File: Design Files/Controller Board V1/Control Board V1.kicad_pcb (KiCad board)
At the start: 4 copper layers, 75 x 125 mm, 78 parts, among them J1 XT30PW-F, J10 SM04B-GHS-TB_LF__SN_-, J11 SM04B-GHS-TB_LF__SN_-, J2 XT30UPB-M, J3 XT30UPB-M, J4 XT30UPB-M, J5 XT30UPB-M, J6 XT30UPB-M, J7 XT30UPB-M, J8 SM04B-GHS-TB_LF__SN_-, J9 SM04B-GHS-TB_LF__SN_-, Q1 LMG5200, U1 LMR51420XDDCR, U2 INA219BIDR, U3 INA219BIDR, U4 INA219BIDR, U5 SC0917, U6 TCA39306DCUR

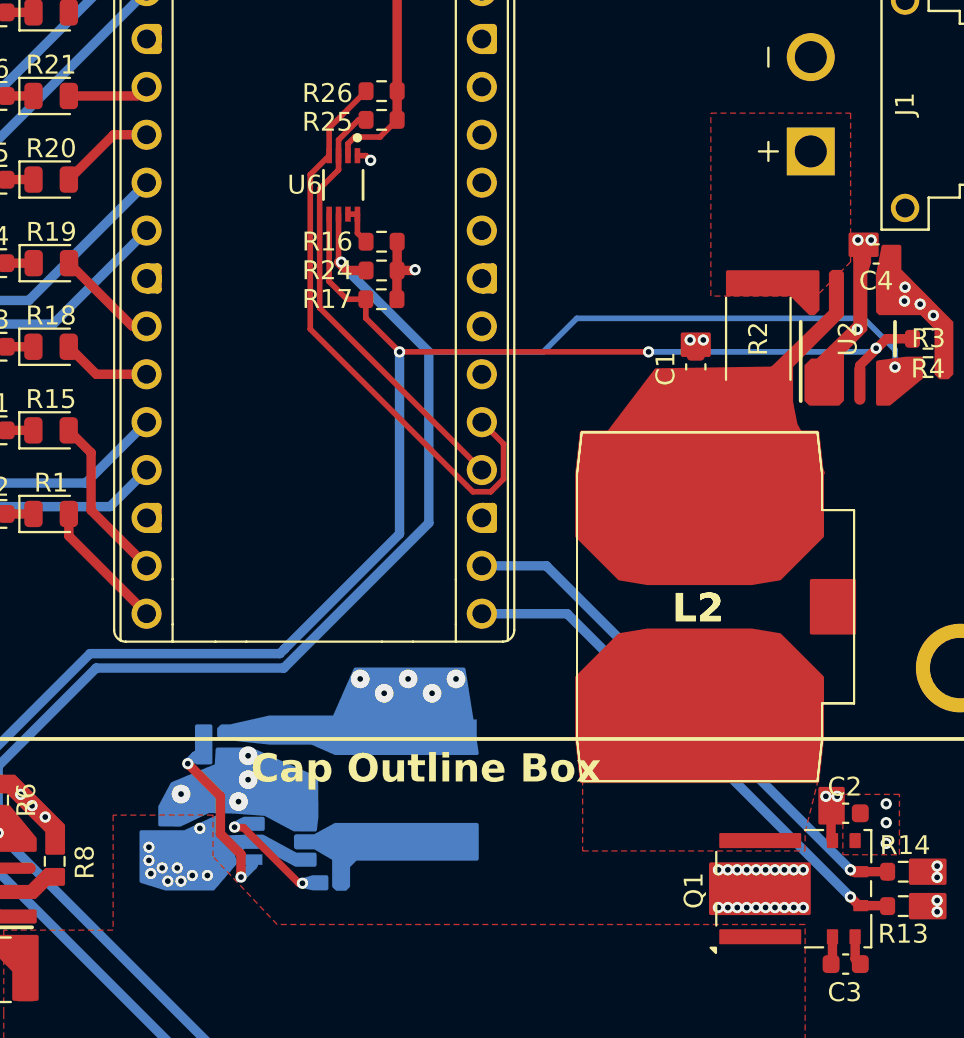
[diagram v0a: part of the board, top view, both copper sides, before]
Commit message: cleaning up stuffs
5vpsu and pour to cabbage
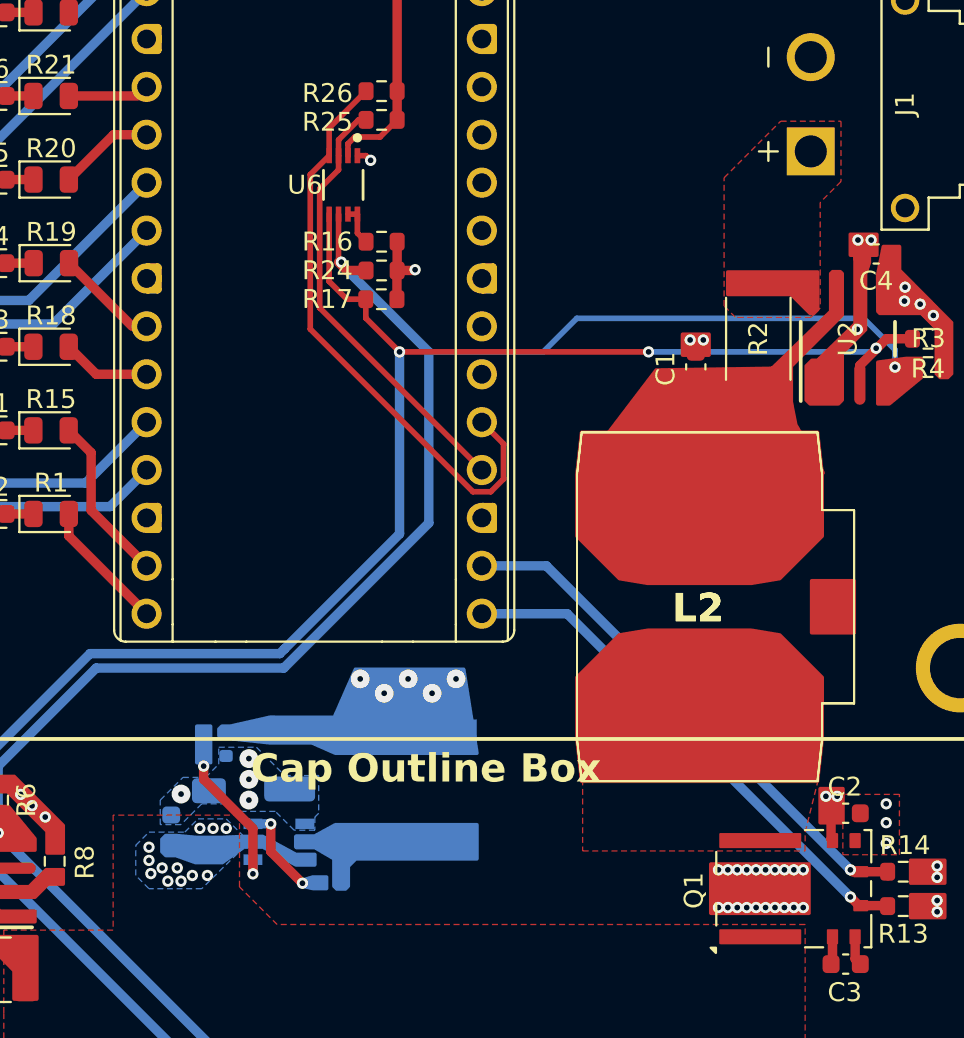
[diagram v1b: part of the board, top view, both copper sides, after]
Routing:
- net Net-(U1-FB): track 9.62 -> 8.34 mm
- net /24V_IN: vias 10 -> 12
- added copper zone on B.Cu, net /24V_IN
- added copper zone on B.Cu, net A_GND
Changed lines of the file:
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@@
-	(gr_poly
-		(pts
-			(xy 88.138 99.314) (xy 89.916 99.314) (xy 93.37421 100.841278) (xy 93.379891 102.062557) (xy 93.382903 102.926902)
-			(xy 93.307662 103.570302) (xy 92.205671 103.561782) (xy 90.666976 102.74158) (xy 89.056591 102.620162)
-			(xy 87.663481 102.58821) (xy 86.148952 103.310327) (xy 85.09 103.297546) (xy 85.09 102.362) (xy 85.739966 101.143976)
-			(xy 86.73687 100.728599) (xy 88.085248 100.172633)
-		)
-		(stroke
-			(width 0.2)
-			(type solid)
-		)
-		(fill solid)
-		(layer "B.Cu")
-		(net 22)
-	)
 	(gr_poly
 		(pts
 			(xy 93.915581 106.086925) (xy 93.190581 106.086925) (xy 92.515581 106.286925) (xy 92.515581 106.536925)
 			(xy 93.190581 106.686925) (xy 93.915581 106.686925)
-		)
-		(stroke
-			(width 0.2)
-			(type solid)
-		)
-		(fill solid)
-		(layer "B.Cu")
-		(net 2)
-	)
-	(gr_poly
-		(pts
-			(xy 84.1 106.3) (xy 85.4 106.7) (xy 87.9 106.7) (xy 89.1 105.3) (xy 88.1 102.9) (xy 86.4 103.7) (xy 84.1 103.7)
-		)
-		(stroke
-			(width 0.2)
-			(type solid)
-		)
-		(fill solid)
-		(layer "B.Cu")
-		(net 3)
-	)
-	(gr_poly
-		(pts
-			(xy 89.540581 102.986925) (xy 88.915581 103.311925) (xy 88.915581 103.561925) (xy 89.165581 103.561925)
-			(xy 89.540581 103.536925) (xy 90.540581 103.536925) (xy 90.540581 102.986925)
 		)
 		(stroke
@@
 	)
 	(segment
-		(start 92.455755 106.411099)
-		(end 92.615581 106.411099)
-		(width 0.4)
+		(start 90.961575 103.261575)
+		(end 90.961575 104.732919)
+		(width 0.5)
 		(layer "F.Cu")
 		(net 2)
 	)
 	(segment
-		(start 89.040581 103.462751)
-		(end 89.507407 103.462751)
-		(width 0.4)
+		(start 90.961575 104.732919)
+		(end 92.640581 106.411925)
+		(width 0.5)
 		(layer "F.Cu")
 		(net 2)
 	)
-	(segment
-		(start 89.038929 103.436925)
-		(end 89.065581 103.463577)
-		(width 0.2)
-		(layer "F.Cu")
+	(via
+		(at 92.640581 106.411925)
+		(size 0.6)
+		(drill 0.3)
+		(layers "F.Cu" "B.Cu")
 		(net 2)
 	)
-	(segment
-		(start 89.507407 103.462751)
-		(end 92.455755 106.411099)
-		(width 0.4)
-		(layer "F.Cu")
+	(via
+		(at 90.961575 103.261575)
+		(size 0.6)
+		(drill 0.3)
+		(layers "F.Cu" "B.Cu")
 		(net 2)
 	)
-	(via
-		(at 92.640581 106.411925)
-		(size 0.6)
-		(drill 0.3)
-		(layers "F.Cu" "B.Cu")
+	(segment
+		(start 90.961575 103.261575)
+		(end 90.012631 103.261575)
+		(width 0.5)
+		(layer "B.Cu")
 		(net 2)
 	)
 	(via
-		(at 89.038929 103.436925)
-		(size 0.6)
-		(drill 0.3)
-		(layers "F.Cu" "B.Cu")
-		(net 2)
-	)
-	(via
 		(at 86.2 106.3)
 		(size 0.6)
@@
 	)
 	(via
+		(at 87.9 103.5)
+		(size 0.6)
+		(drill 0.3)
+		(layers "F.Cu" "B.Cu")
+		(free yes)
+		(net 3)
+	)
+	(via
 		(at 85.2 105.6)
 		(size 0.6)
@@
 	(via
 		(at 87.6 106)
+		(size 0.6)
+		(drill 0.3)
+		(layers "F.Cu" "B.Cu")
+		(free yes)
+		(net 3)
+	)
+	(via
+		(at 88.6 103.5)
 		(size 0.6)
 		(drill 0.3)
@@
 	)
 	(via blind
-		(at 89.758581 100.919925)
+		(at 89.8 100.9)
 		(size 1)
 		(drill 0.3)
@@
 	)
 	(via blind
-		(at 89.248735 102.082033)
+		(at 89.8 102)
 		(size 1)
 		(drill 0.3)
@@
 	)
 	(via blind
-		(at 89.758581 99.649925)
+		(at 89.8 99.8)
 		(size 1)
 		(drill 0.3)
@@
 	)
 	(segment
-		(start 89.379778 104.879778)
-		(end 88.288929 103.788929)
+		(start 87.4 100.9)
+		(end 87.4 100.2)
 		(width 0.5)
 		(layer "F.Cu")
@@
 	)
 	(segment
-		(start 88.288929 103.788929)
-		(end 88.288929 101.79877)
+		(start 90.012631 105.912631)
+		(end 90.012631 103.512631)
 		(width 0.5)
 		(layer "F.Cu")
@@
 	)
 	(segment
-		(start 88.288929 101.79877)
-		(end 86.558987 100.068828)
+		(start 90.012631 103.512631)
+		(end 87.4 100.9)
 		(width 0.5)
 		(layer "F.Cu")
 		(net 28)
 	)
-	(segment
-		(start 89.379778 106.085045)
-		(end 89.379778 104.879778)
-		(width 0.5)
-		(layer "F.Cu")
+	(via
+		(at 87.4 100.2)
+		(size 0.6)
+		(drill 0.3)
+		(layers "F.Cu" "B.Cu")
 		(net 28)
 	)
 	(via
-		(at 86.558987 100.068828)
+		(at 90.012631 105.912631)
 		(size 0.6)
 		(drill 0.3)
@@
 		(net 28)
 	)
-	(via
-		(at 89.379778 106.085045)
-		(size 0.6)
-		(drill 0.3)
-		(layers "F.Cu" "B.Cu")
+	(segment
+		(start 87.4 100.2)
+		(end 87.4 99.668494)
+		(width 0.5)
+		(layer "B.Cu")
 		(net 28)
 	)
 	(segment
-		(start 86.558987 100.068828)
-		(end 86.96624 99.661575)
-		(width 0.5)
-		(layer "B.Cu")
-		(net 28)
-	)
-	(segment
-		(start 86.96624 99.661575)
+		(start 87.4 99.668494)
 		(end 87.393081 99.661575)
-		(width 0.5)
-		(layer "B.Cu")
-		(net 28)
-	)
-	(segment
-		(start 90.012631 105.452192)
-		(end 90.012631 105.161577)
-		(width 0.5)
-		(layer "B.Cu")
-		(net 28)
-	)
-	(segment
-		(start 89.379778 106.085045)
-		(end 90.012631 105.452192)
 		(width 0.5)
 		(layer "B.Cu")
@@
 		(end 90.040581 105.161925)
 		(width 0.2)
+		(layer "B.Cu")
+		(net 28)
+	)
+	(segment
+		(start 90.012631 105.912631)
+		(end 90.012631 105.161577)
+		(width 0.5)
 		(layer "B.Cu")
 		(net 28)
@@
 			(pts
 				(xy 76.8 108.9) (xy 76.8 113.3) (xy 76.8 122.1) (xy 83.6 122.1) (xy 99.5 122.1) (xy 99.5 120.5)
-				(xy 99.9 119.9) (xy 101 118.8) (xy 119.3 118.8) (xy 119.3 108.6) (xy 91.3 108.6) (xy 87.9 105) (xy 87.9 102.8)
-				(xy 82.6 102.8) (xy 82.6 108.9)
+				(xy 99.9 119.9) (xy 101 118.8) (xy 119.3 118.8) (xy 119.3 108.6) (xy 91.3 108.6) (xy 89.3 106.6)
+				(xy 89.3 102.8) (xy 82.6 102.8) (xy 82.6 108.9)
 			)
 		)
@@
 		(polygon
 			(pts
-				(xy 74.37 114.71) (xy 65.82 114.71) (xy 65.82 114.71) (xy 65.82 107.54) (xy 65.82 107.54) (xy 74.38 107.54)
-				(xy 74.362316 112.442316) (xy 74.37 112.45) (xy 74.37 114.71)
+				(xy 74.37 114.71) (xy 65.82 114.71) (xy 65.82 107.54) (xy 74.38 107.54) (xy 74.362316 112.442316)
+				(xy 74.37 112.45)
 			)
 		)
@@
 			(thermal_gap 0.5)
 			(thermal_bridge_width 0.5)
-			(smoothing chamfer)
-			(radius 0.5)
 		)
 		(polygon
 			(pts
-				(xy 119.9 75.27) (xy 114.3 75.27) (xy 114.3 65.57) (xy 121.71 65.57) (xy 121.71 73.46)
+				(xy 120.1 75.9) (xy 119.595122 76.4) (xy 115.6 76.4) (xy 115 75.8) (xy 115 69) (xy 118 66) (xy 121.2 66)
+				(xy 121.2 69.2) (xy 120.1 70.3)
 			)
 		)
@@
 			)
 		)
+	)
+	(zone
+		(net 3)
+		(net_name "/24V_IN")
+		(layer "B.Cu")
+		(hatch none 0.25)
+		(priority 4)
+		(connect_pads yes
+			(clearance 0)
+		)
+		(min_thickness 0.25)
+		(filled_areas_thickness no)
+		(fill yes
+			(thermal_gap 0.5)
+			(thermal_bridge_width 0.5)
+			(island_removal_mode 1)
+			(island_area_min 10)
+		)
+		(polygon
+			(pts
+				(xy 84.5 103.7) (xy 86.4 103.7) (xy 87.1 103) (xy 88.6 103) (xy 89.540581 103.936925) (xy 89.540581 104.486925)
+				(xy 87.3 106.7) (xy 84.5 106.7) (xy 83.8 106) (xy 83.8 104.4)
+			)
+		)
+	)
+	(zone
+		(net 22)
+		(net_name "A_GND")
+		(layer "B.Cu")
+		(hatch none 0.25)
+		(priority 4)
+		(connect_pads yes
+			(clearance 0)
+		)
+		(min_thickness 0.25)
+		(filled_areas_thickness no)
+		(fill yes
+			(thermal_gap 0.5)
+			(thermal_bridge_width 0.5)
+			(island_removal_mode 1)
+			(island_area_min 10)
+		)
+		(polygon
+			(pts
+				(xy 88.6 102.2) (xy 87.3 102.2) (xy 86.2 103.3) (xy 85.1 103.3) (xy 85.1 102) (xy 86.3 100.8) (xy 87.5 100.8)
+				(xy 88.2 100.1) (xy 88.2 99.2) (xy 90.2 99.2) (xy 91.7 100.7) (xy 93.5 100.7) (xy 93.5 102.7) (xy 93.3 102.9)
+				(xy 93.3 103.6) (xy 92.2 103.6) (xy 91.2 102.6) (xy 89 102.6)
+			)
+		)
